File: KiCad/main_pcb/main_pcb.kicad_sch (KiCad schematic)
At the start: 5 parts

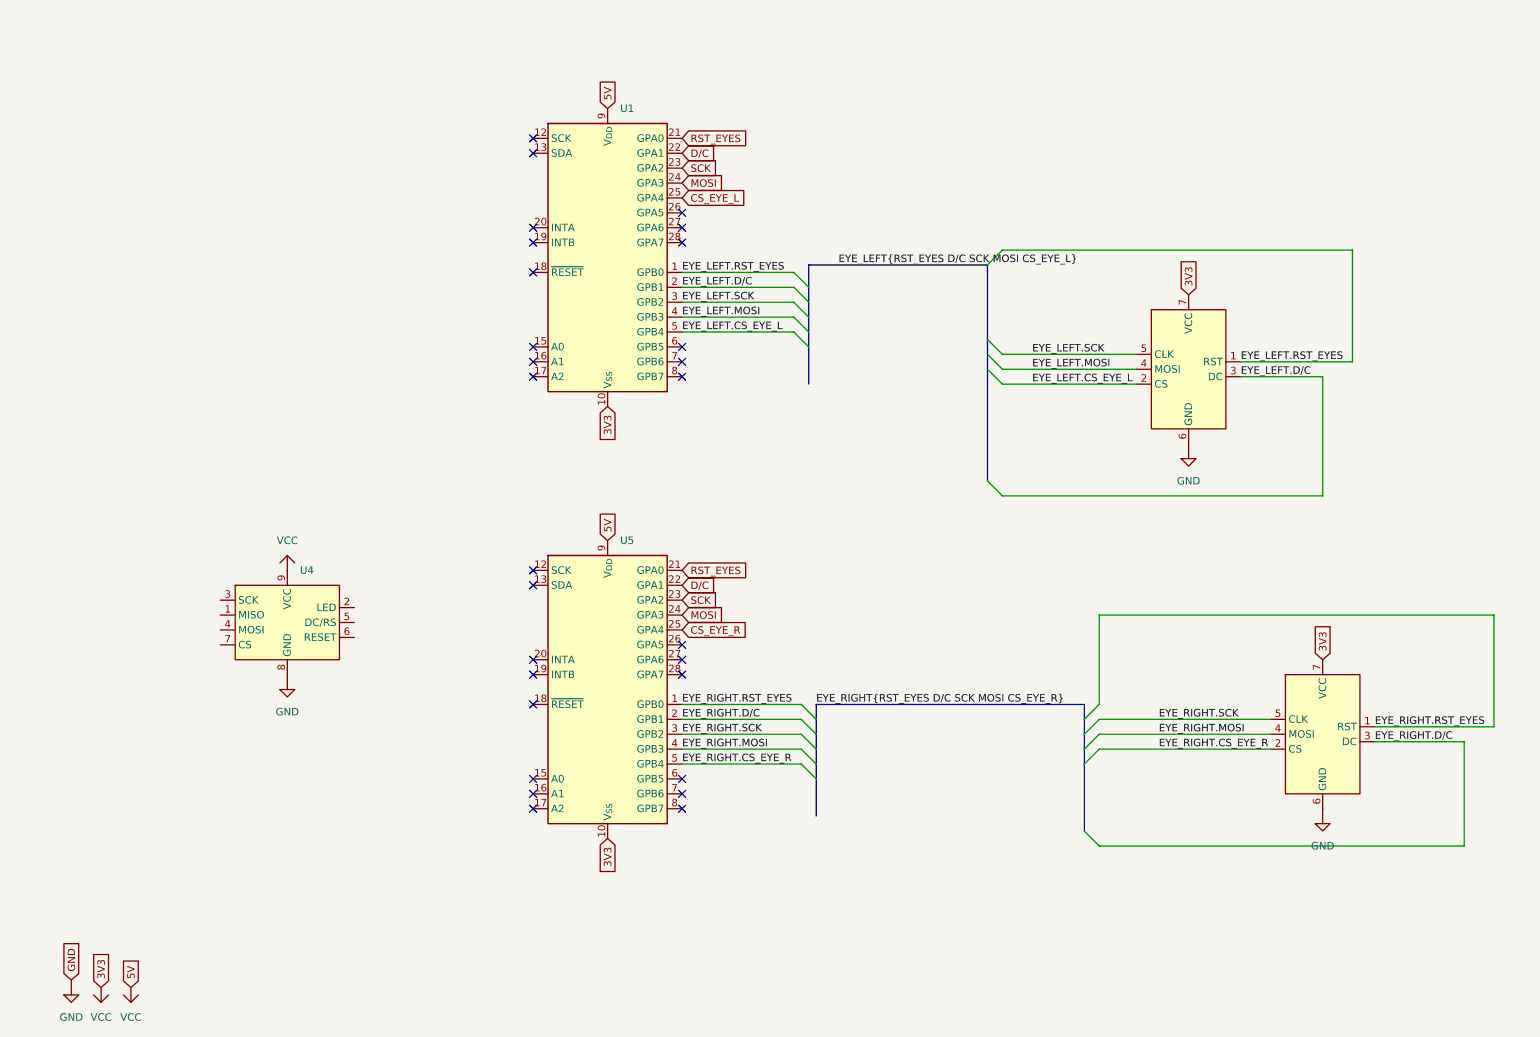
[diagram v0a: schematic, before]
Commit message: feat(KiCad): Adds circuit for the screens
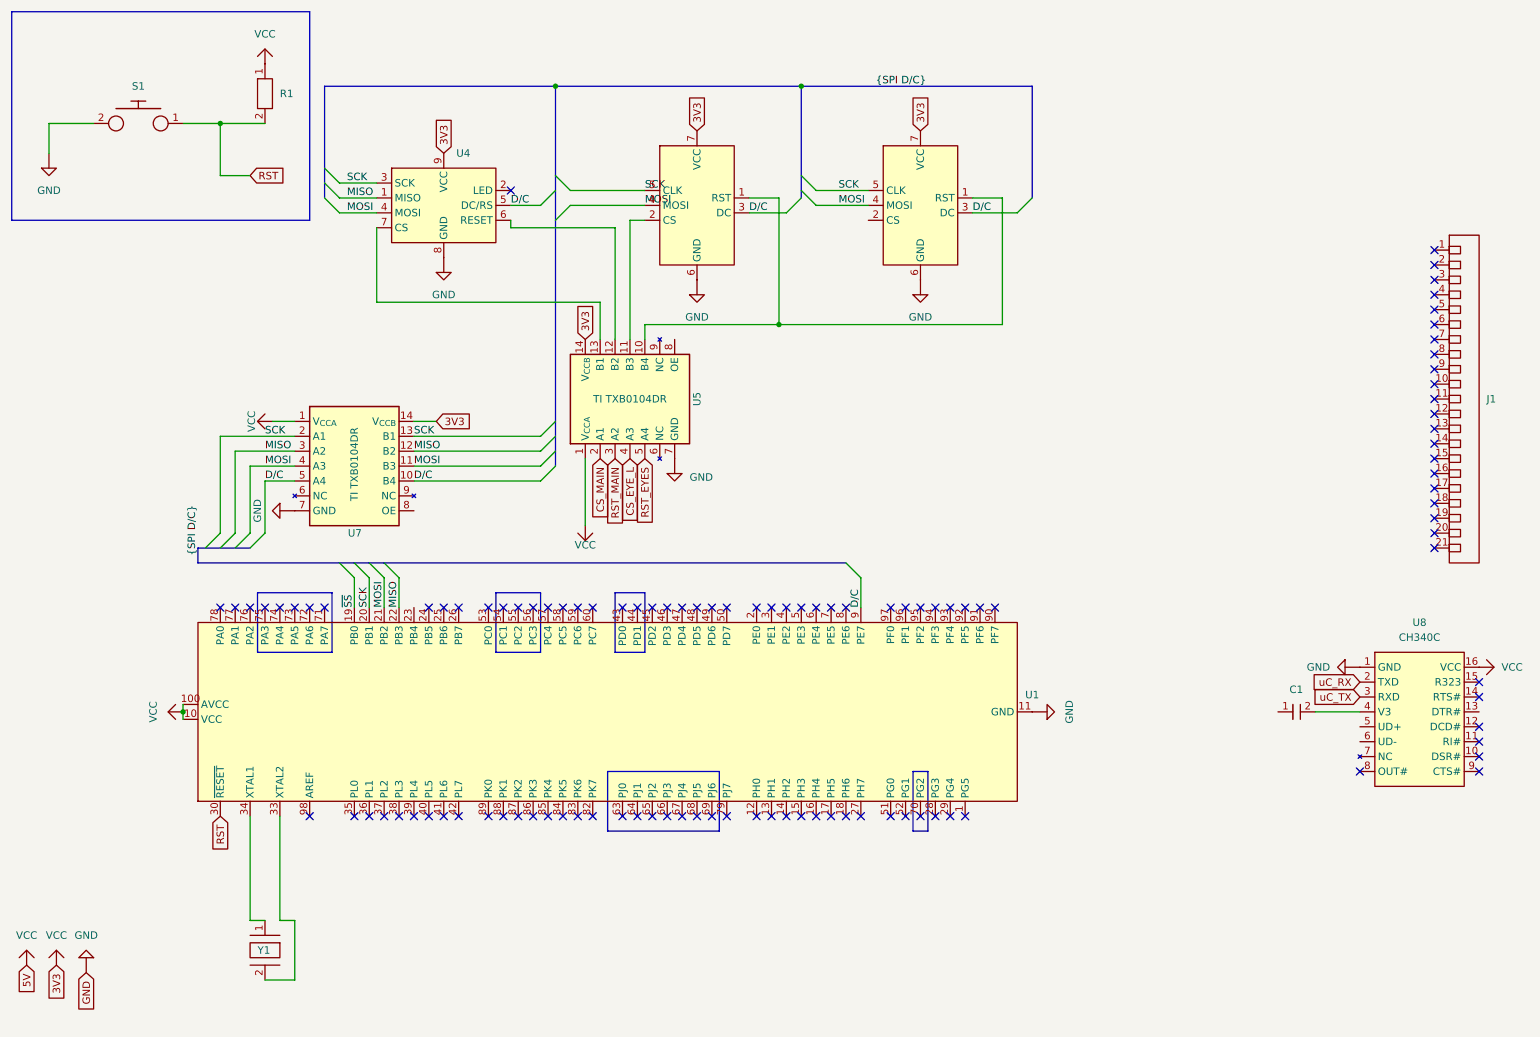
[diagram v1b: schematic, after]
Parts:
- removed U1, U5: (no value), symbol Lily's_Pad:Logic_Converter
- added C1: (no value), symbol Lily's_Pad:Capacitor
- added J1: (no value), symbol Lily's_Pad:Header_21
- added R1: (no value), symbol Lily's_Pad:Resistor
- added S1: (no value), symbol Lily's_Pad:Push-button_Switch
- added U1: (no value), symbol Lily's_Pad:ATmega_2560
- added U5, U7: TI TXB0104DR, symbol Lily's_Pad:TI TXB0104DR
- added U8: CH340C, symbol Lily's_Pad:CH340C
- added Y1: (no value), symbol Lily's_Pad:Crystal
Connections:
- net EYE_LEFT.D/C is gone; now on net D/C: U2.3 (DC)
- net EYE_LEFT.MOSI is gone; now on net MOSI: U2.4 (MOSI)
- net EYE_LEFT.SCK is gone; now on net SCK: U2.5 (CLK)
- net EYE_RIGHT.D/C is gone; now on net D/C: U3.3 (DC)
- net EYE_RIGHT.MOSI is gone; now on net MOSI: U3.4 (MOSI)
- net EYE_RIGHT.RST_EYES is gone; now on an unnamed net: U3.1 (RST)
- net EYE_RIGHT.SCK is gone; now on net SCK: U3.5 (CLK)
- net CS_EYE_L: now also U5.4 (A3)
- net D/C: now also U4.5 (DC/RS), U1.9 (PE7), U7.10 (B4), U7.5 (A4)
- net GND: now also S1.2, U1.11 (GND), U1.32 (GND), U1.62 (GND), U1.81 (GND), U1.99 (GND), U5.7 (GND), U7.7 (GND), U8.1 (GND); no longer U4.8 (GND)
- net MOSI: now also U4.4 (MOSI), U1.21 (PB2), U7.11 (B3), U7.4 (A3)
- net RST_EYES: now also U5.5 (A4)
- net SCK: now also U4.3 (SCK), U1.20 (PB1), U7.13 (B1), U7.2 (A1)
- net VCC: now also R1.1, U1.10 (VCC), U1.100 (AVCC), U1.31 (VCC), U1.61 (VCC), U1.80 (VCC), U5.1 (V_{CCA}), U5.14 (V_{CCB}), U7.1 (V_{CCA}), U7.14 (V_{CCB}), U8.16 (VCC); no longer U4.9 (VCC)
- net MISO: now reaches U4.1 (MISO)
- net MISO: now also U1.22 (PB3), U7.12 (B2), U7.3 (A2)
- net at U4.6 (RESET): now also U5.12 (B2)
- net at U4.7 (CS): now also U5.13 (B1)
- net EYE_LEFT.CS_EYE_L: no longer names the net of U2.2 (CS)
- net EYE_LEFT.RST_EYES: no longer names the net of U2.1 (RST)
- net EYE_LEFT.RST_EYES: now also U5.10 (B4)
- net EYE_RIGHT.CS_EYE_R: no longer names the net of U3.2 (CS)
- net EYE_RIGHT.CS_EYE_R: now also U5.11 (B3)
- new net: C1.2, U8.4 (V3)
- new net: U1.34 (XTAL1), Y1.1
- new net: U1.33 (XTAL2), Y1.2
- new net CS_MAIN: U5.2 (A1)
- new net RST: R1.2, S1.1, U1.30 (~{RESET})
- new net RST_MAIN: U5.3 (A2)
- new net uC_RX: U8.2 (TXD)
- new net uC_TX: U8.3 (RXD)
- new net ~{SS}: U1.19 (PB0)
- no-connect marks 28 -> 110
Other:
- company: (none) -> Lily's Pad
- title: (none) -> Main PCB
